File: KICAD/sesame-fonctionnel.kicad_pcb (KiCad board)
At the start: 2 copper layers, 160 x 100 mm, 278 parts, among them J1 CXS70-14-C, J2 CXS70-14-C, J7 CXS70-14-C, J8 CXS70-14-C, J9 Conn_02x16_Odd_Even, Q1 BC847, Q10 BC857, Q11 SQM120, Q12 BC847, Q13 BC847, Q2 BC847, Q3 BC847, Q4 BC847, Q5 BC847, Q6 SQM120, Q7 BC857, Q8 SQM120, Q9 SQM120, U1 AD8030, U10 LT6016, U11 AD8030, U12 UCC27284-Q1, U13 AD8030, U14 AD8030, U15 LT8365, U16 LM4040DBZ-2.5, U17 UCC27284-Q1, U2 LM2903, U3 CD4053BM96, U4 4011, U5 CD4053BM96, U6 CD4053BM96, U7 AD8030, U8 LT6016, U9 AD8030

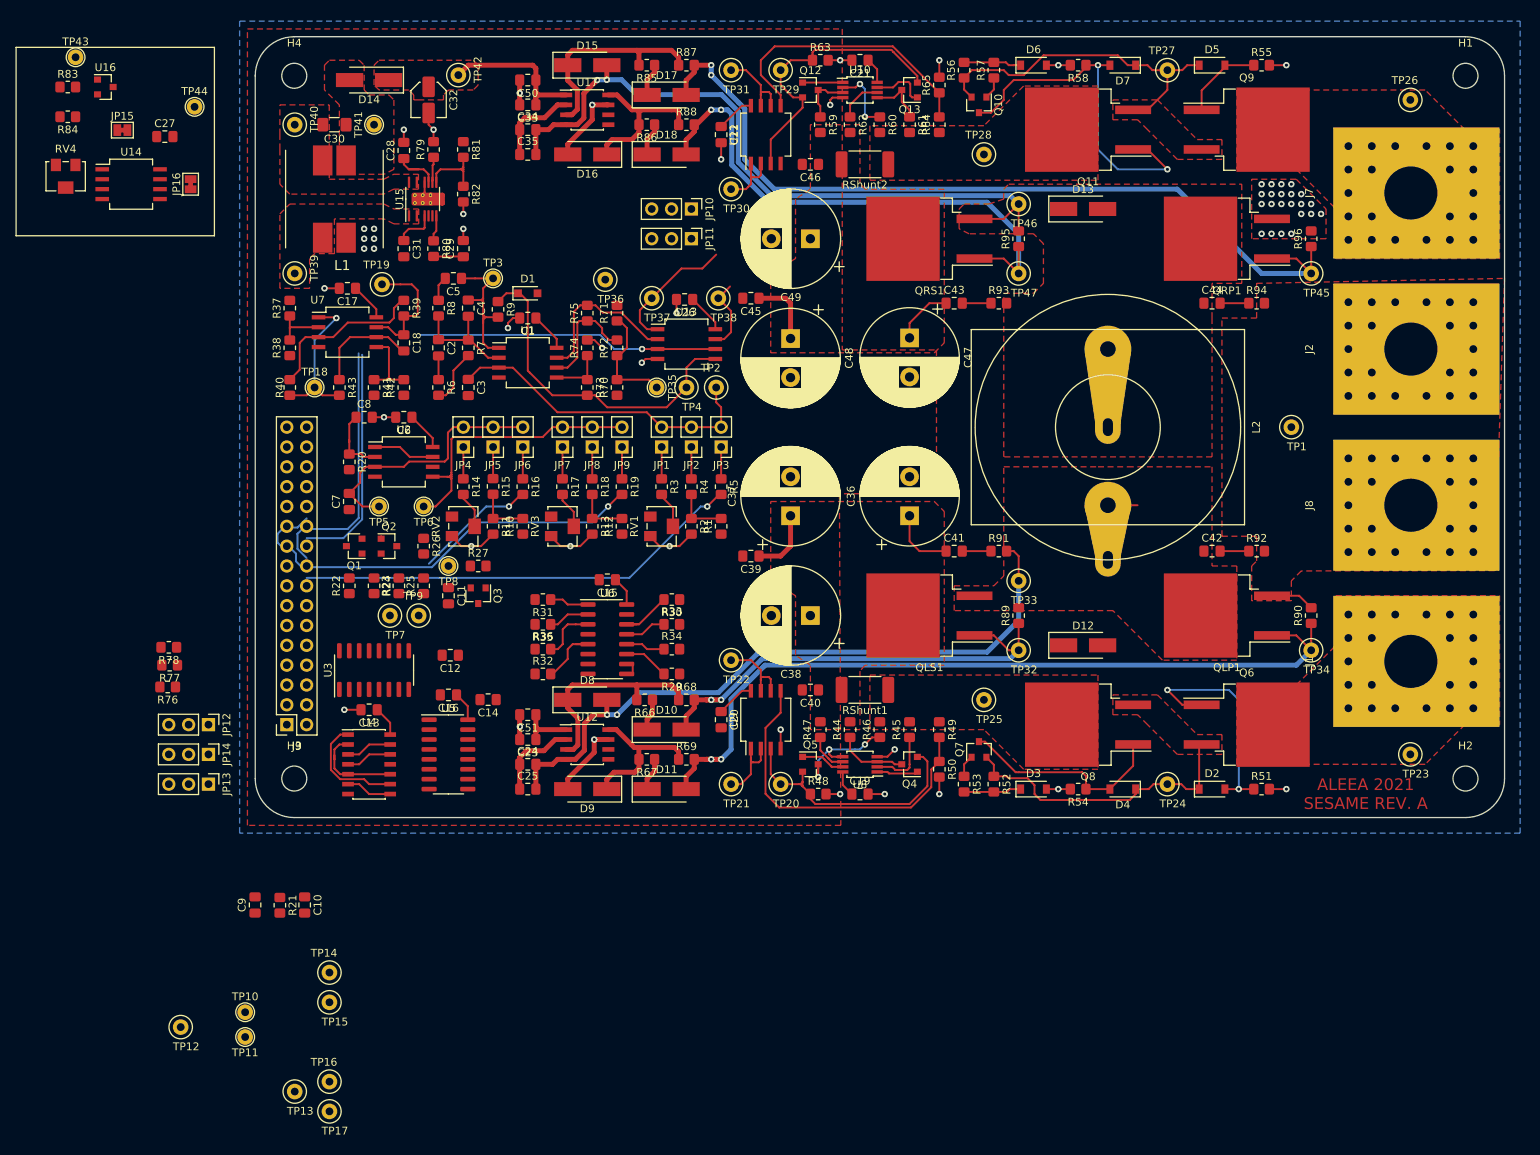
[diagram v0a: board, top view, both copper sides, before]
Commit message: test w/ layers indicator
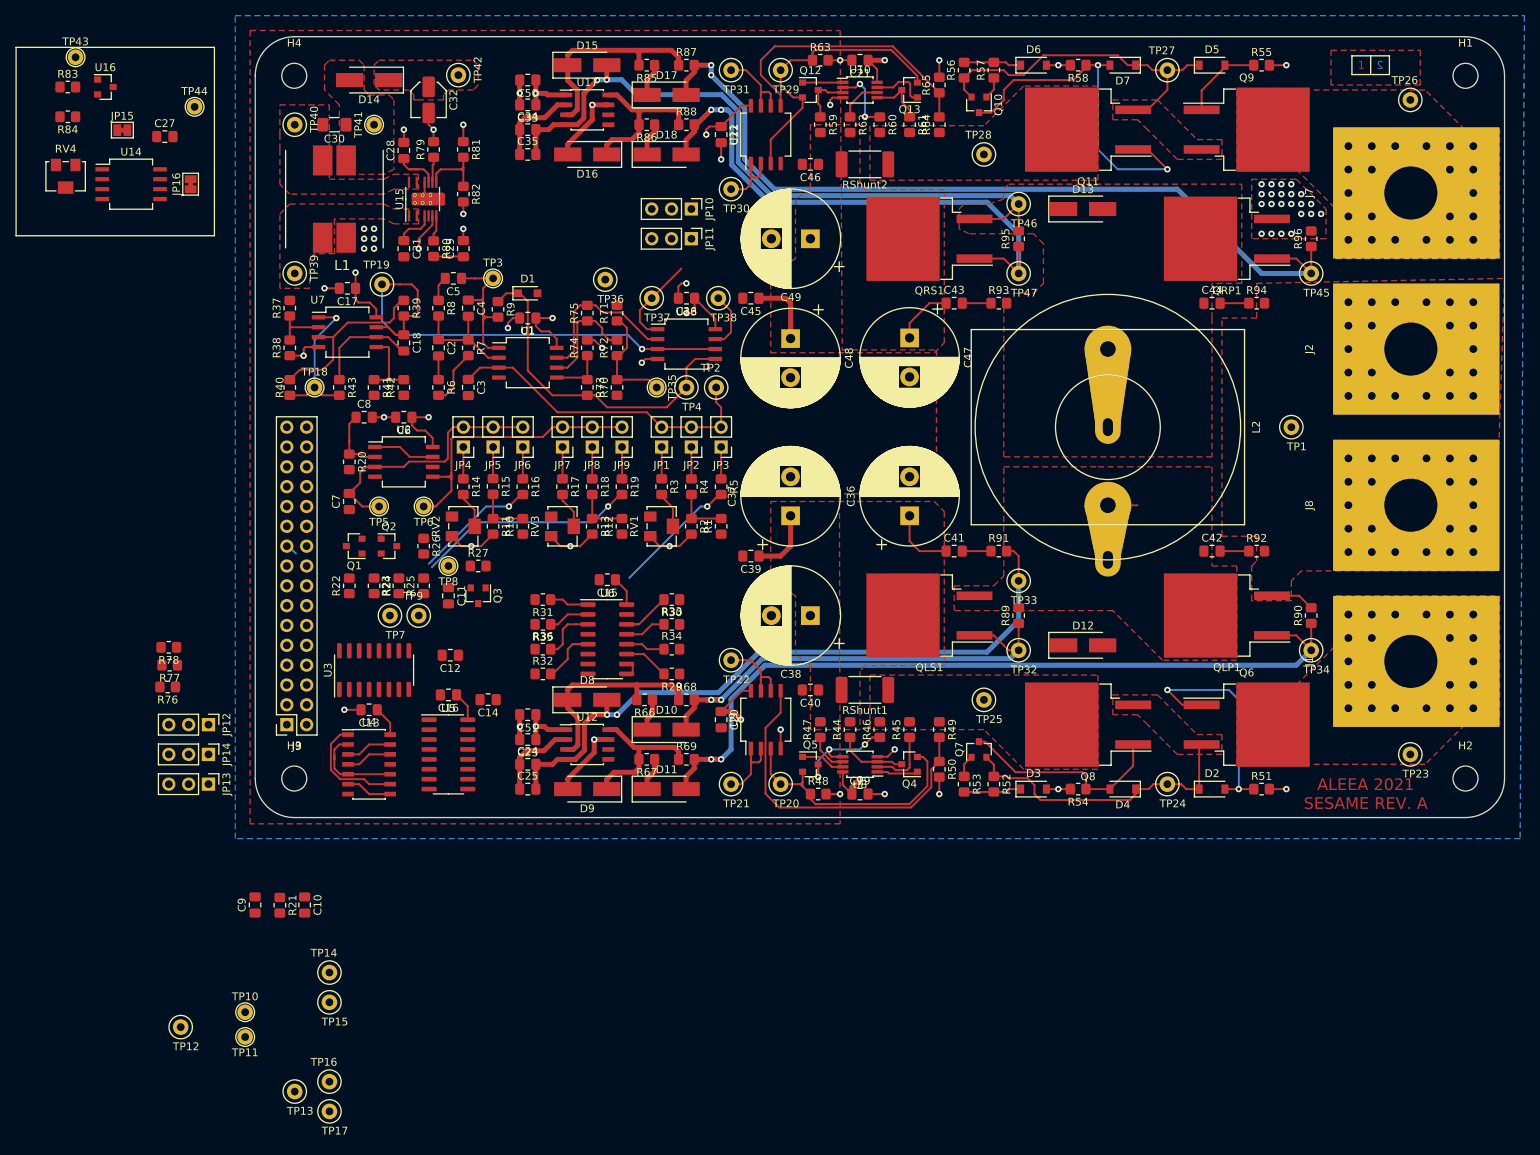
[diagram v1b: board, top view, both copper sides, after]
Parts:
- added REF**: Layer_indicator_2L, Sesame_footprint:Layer_indicator, F.Cu at (222.9, 63.6)
- moved C26 0.28 mm to (135.2, 93.5)
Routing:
- net /Current_Thres: track 88.9 -> 28.2 mm
- net /Ext_Setpoint: track 57.5 -> 16.2 mm
- net /INT EXT CONFIG/~Ext_PWM: track 29.2 -> 0.00 mm
- net VCC: track 74.9 -> 90.4 mm, vias 0 -> 12
- net /PWM GEN/Ramp: track 54.6 -> 65.0 mm
- net GND: track 117.4 -> 125.1 mm, vias 59 -> 60
- net /~INT_PWM_Freewheel: track 16.9 -> 11.7 mm
- net /INT_PWM_Power: track 9.54 -> 7.41 mm
- net Net-(R39-Pad1): track 21.6 -> 23.1 mm
- added copper zone on F.Cu, net (none)
- added copper zone on In1.Cu, net VCC
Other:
- copper layers 2 -> 4
